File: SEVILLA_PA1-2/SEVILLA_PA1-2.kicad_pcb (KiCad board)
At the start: 2 copper layers, 42.5 x 36.5 mm, 8 parts, among them SW1 SW_DIP_x02, U1 74LS04, U2 74LS08, U3 74LS32

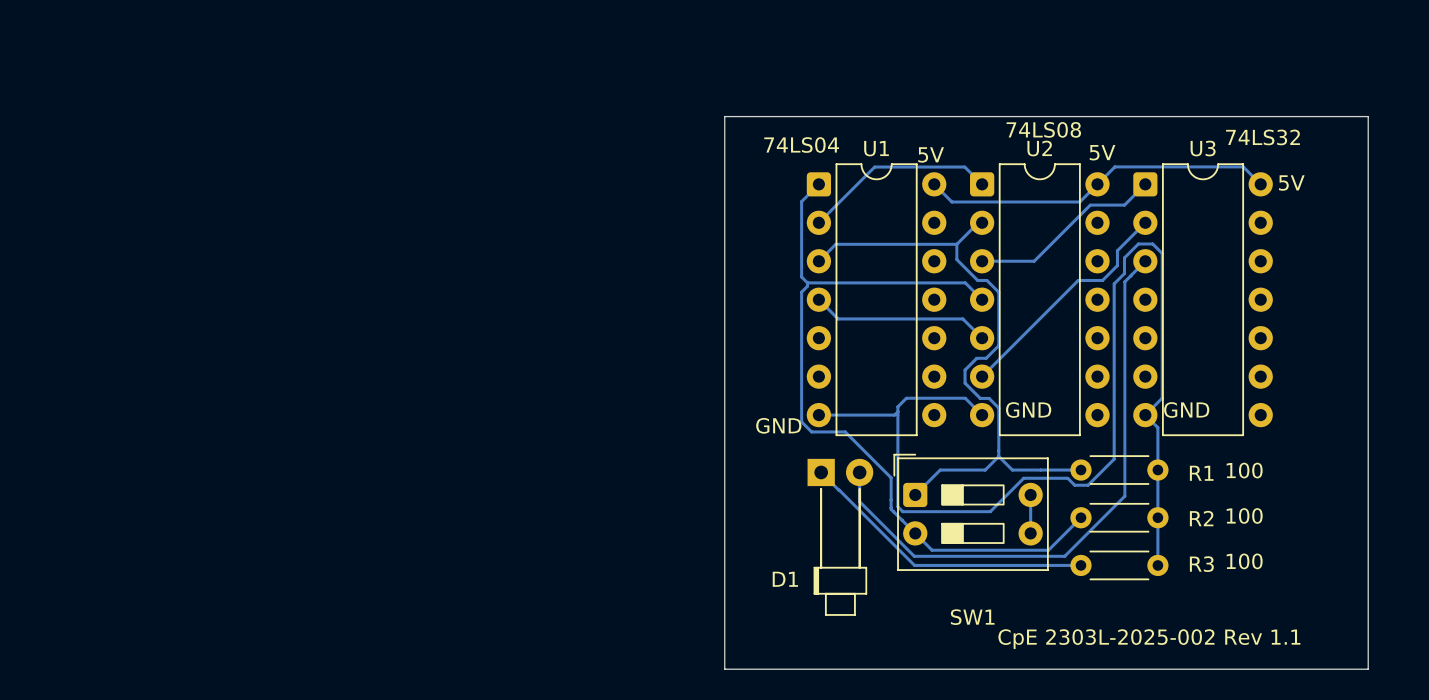
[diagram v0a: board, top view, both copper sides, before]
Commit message: Refactor code structure and remove redundant sections for improved readability and maintainability
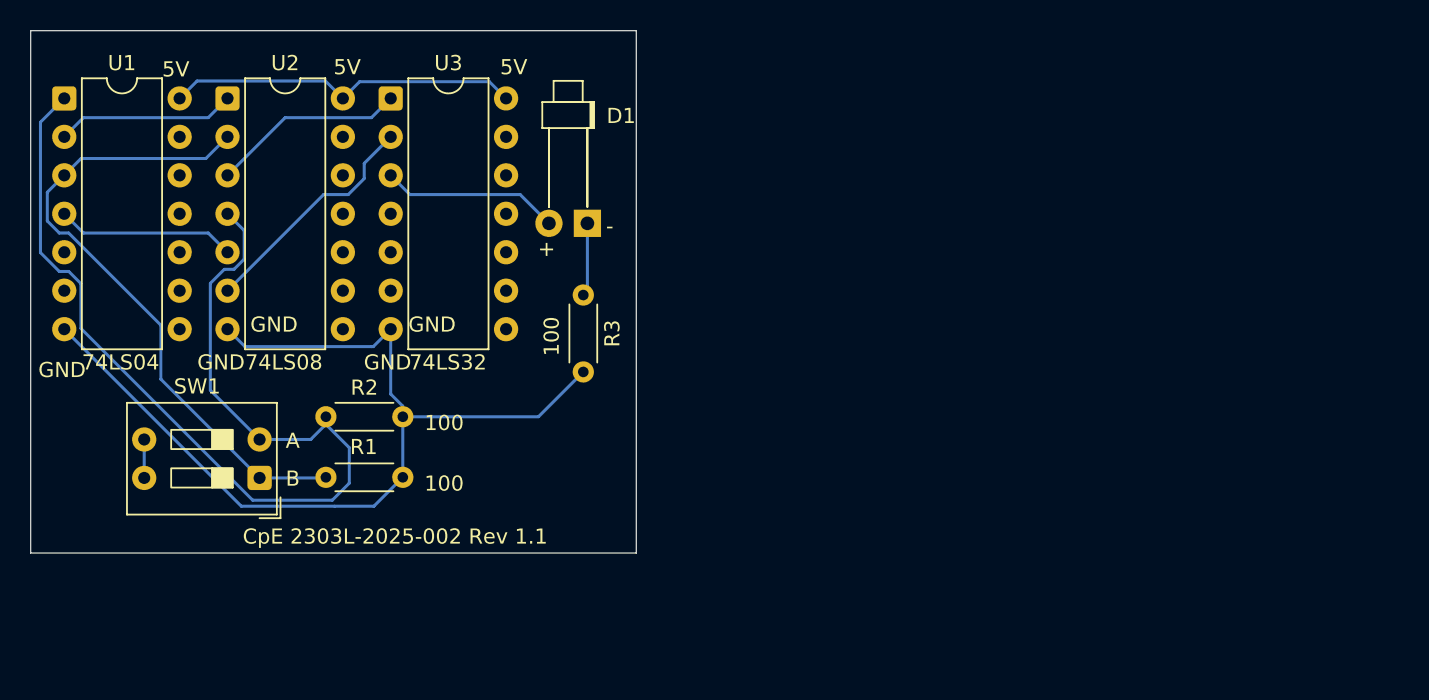
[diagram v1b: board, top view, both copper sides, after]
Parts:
- moved R2 50.3 mm to (142.2, 118.3)
- moved U1 50.2 mm to (124.9, 97.3)
- moved U2 50.2 mm to (135.7, 97.3)
- moved U3 50.2 mm to (146.4, 97.3)
- moved R1 49.9 mm to (142.2, 122.3)
- moved SW1 43.3 mm to (137.8, 122.4), turned to 180 degrees
- moved R3 37.4 mm to (159.2, 110.3), turned to -90 degrees
- moved D1 22.6 mm to (159.4, 105.5), turned to 180 degrees
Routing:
- net Net-(D1-A): track 38.7 -> 11.8 mm
- net Net-(R2-Pad1): track 52.5 -> 67.5 mm
- net Net-(D1-K): track 19.7 -> 4.85 mm
- net GND: track 72.5 -> 63.0 mm
- net Net-(U1-Pad2): track 12.8 -> 11.8 mm
- net Net-(R1-Pad1): track 42.3 -> 43.0 mm
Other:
- board size 42.5 x 36.5 mm -> 40 x 34.5 mm
- board text added: "+"
- board text added: "-"
- board text added: "A"
- board text added: "B"
